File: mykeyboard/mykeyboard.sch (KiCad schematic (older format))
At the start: 2 parts

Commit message: try to select PATH
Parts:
- removed U?: GL850A, symbol Switch:GL850A
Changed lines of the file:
@@
 EESchema Schematic File Version 4
+LIBS:mykeyboard-cache
 EELAYER 26 0
 EELAYER END
@@
 $EndDescr
 $Comp
-L Switch:GL850A U?
-U 1 1 5BE85F64
-P 3000 4200
-F 0 "U?" H 2975 5465 50  0000 C CNN
-F 1 "GL850A" H 2975 5374 50  0000 C CNN
-F 2 "" H 2300 5400 50  0001 C CNN
-F 3 "" H 2300 5400 50  0001 C CNN
-	1    3000 4200
-	1    0    0    -1
-$EndComp
-$Comp
 L MCU_Microchip_ATmega:ATmega32U4-AU U?

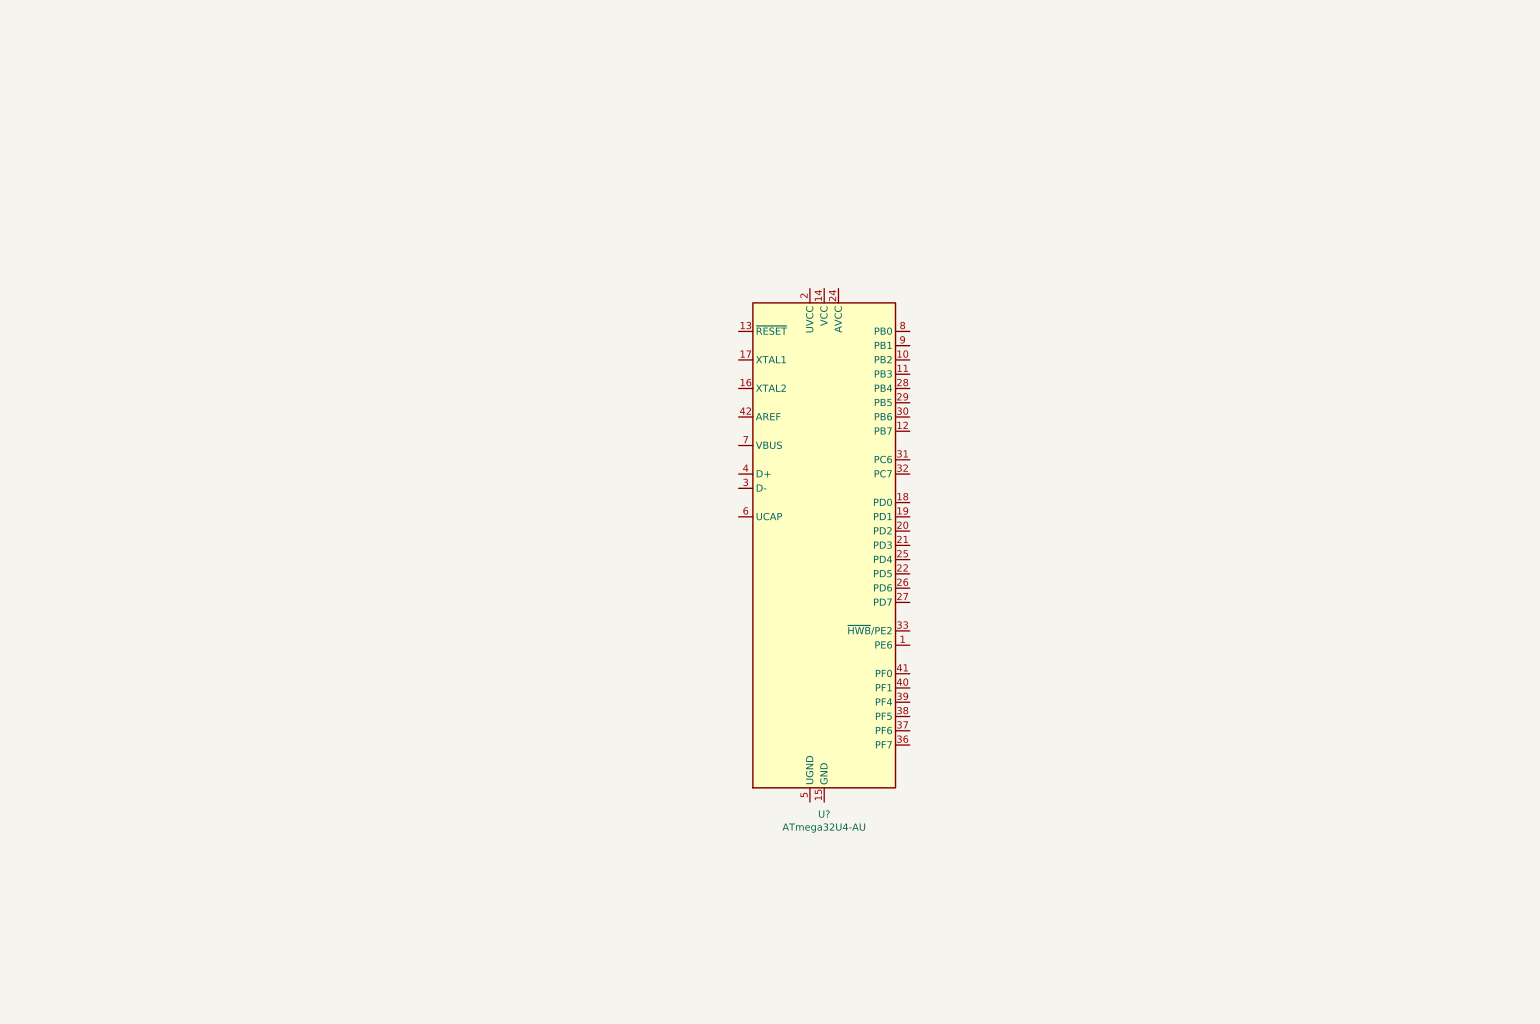
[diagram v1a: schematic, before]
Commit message: 1112,gogogo
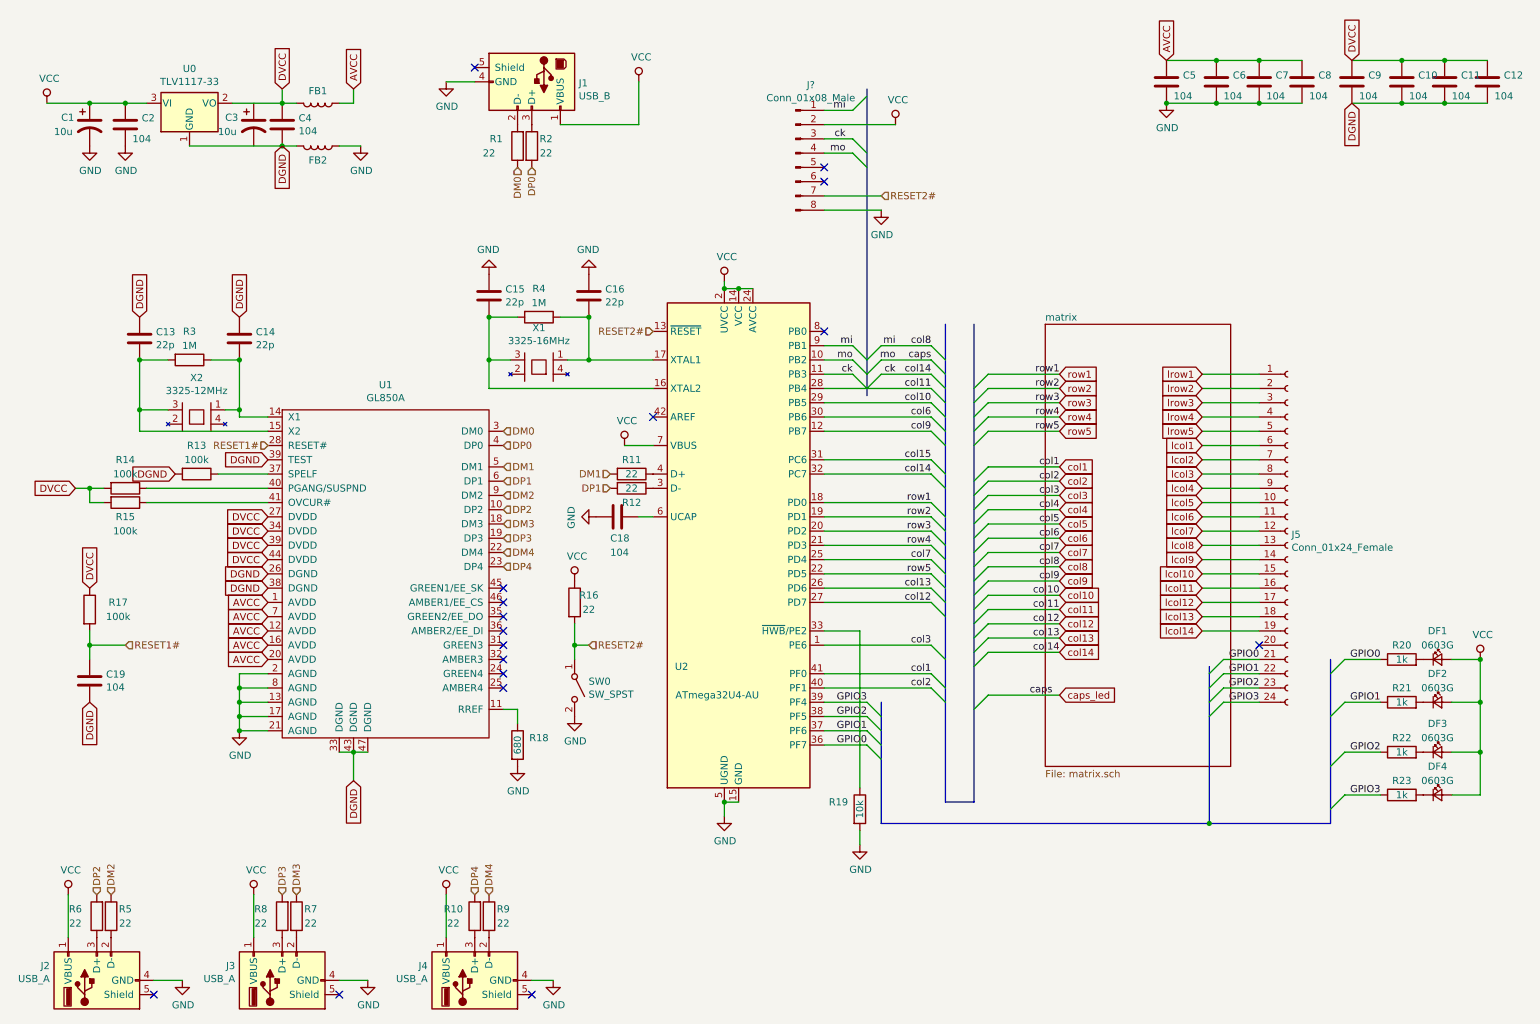
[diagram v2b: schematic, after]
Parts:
- added C1, C3: 10u, symbol Device:CP1
- added C10, C11, C12, C18, C19, C2, C4, C5, C6, C7, C8, C9: 104, symbol Device:C
- added C13, C14, C15, C16: 22p, symbol Device:C
- added DF1, DF2, DF3, DF4: 0603G, symbol Device:LED_Small
- added FB1, FB2: ~, symbol Device:L
- added J1: USB_B, symbol Connector:USB_B
- added J2, J3, J4: USB_A, symbol Connector:USB_A
- added J5: Conn_01x24_Female, symbol Connector:Conn_01x24_Female
- added J?: Conn_01x08_Male, symbol Connector:Conn_01x08_Male
- added R1, R10, R11, R12, R16, R2, R5, R6, R7, R8, R9: 22, symbol Device:R
- added R13, R14, R15, R17: 100k, symbol Device:R
- added R18: 680, symbol Device:R
- added R19: 10k, symbol Device:R
- added R20, R21, R22, R23: 1k, symbol Device:R
- added R3, R4: 1M, symbol Device:R
- added SW0: SW_SPST, symbol Switch:SW_SPST
- added U0: TLV1117-33, symbol Regulator_Linear:TLV1117-33
- added U1: GL850A, symbol mykeyboard-rescue:GL850A-mykeyboardlibs
- added X1: 3325-16MHz, symbol mykeyboard-rescue:3325-16MHz-mykeyboardlibs
- added X2: 3325-12MHz, symbol mykeyboard-rescue:3325-12MHz-mykeyboardlibs
- gave numbers to parts that had none: 1
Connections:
- net col3: now reaches U2.1 (PE6)
- net caps_led: now reaches U2.10 (PB2)
- net caps_led: now also J?.4 (Pin_4)
- net col14: now reaches U2.11 (PB3)
- net col14: now also U2.32 (PC7), J?.3 (Pin_3)
- net col9: now reaches U2.12 (PB7)
- net RESET2#: now reaches U2.13 (~RESET)
- net RESET2#: now also J?.7 (Pin_7), R16.2, SW0.1 (A)
- net VCC: now reaches U2.14 (VCC), U2.34 (VCC)
- net VCC: now also U2.2 (UVCC), U2.24 (AVCC), U2.44 (AVCC), U2.7 (VBUS), C1.1, C2.1, DF1.2 (A), DF2.2 (A), DF3.2 (A), DF4.2 (A), J1.1 (VBUS), J2.1 (VBUS), J3.1 (VBUS), J4.1 (VBUS), J?.2 (Pin_2), R16.1, U0.3 (VI)
- net GND: now reaches U2.15 (GND), U2.23 (GND), U2.35 (GND), U2.43 (GND)
- net GND: now also U2.5 (UGND), C1.2, C15.1, C16.1, C18.2, C2.2, C5.2, C6.2, C7.2, C8.2, FB2.1, J1.4 (GND), J2.4 (GND), J3.4 (GND), J4.4 (GND), J?.8 (Pin_8), R18.2, R19.2, SW0.2 (B), U1.13 (AGND), U1.17 (AGND), U1.2 (AGND), U1.21 (AGND), U1.8 (AGND)
- net at U2.16 (XTAL2): now also C15.2, R4.2, X1.3
- net at U2.17 (XTAL1): now also C16.2, R4.1, X1.1
- net row1: now reaches U2.18 (PD0)
- net row2: now reaches U2.19 (PD1)
- net row3: now reaches U2.20 (PD2)
- net row4: now reaches U2.21 (PD3)
- net row5: now reaches U2.22 (PD5)
- net col7: now reaches U2.25 (PD4)
- net col13: now reaches U2.26 (PD6)
- net col12: now reaches U2.27 (PD7)
- net col11: now reaches U2.28 (PB4)
- net col10: now reaches U2.29 (PB5)
- net at U2.3 (D-): now also R12.1
- net col6: now reaches U2.30 (PB6)
- net col15: now reaches U2.31 (PC6)
- net at U2.33 (~HWB~/PE2): now also R19.1
- net GPIO0: now reaches U2.36 (PF7)
- net GPIO0: now also J5.21 (Pin_21), R20.1
- net GPIO1: now reaches U2.37 (PF6)
- net GPIO1: now also J5.22 (Pin_22), R21.1
- net GPIO2: now reaches U2.38 (PF5)
- net GPIO2: now also J5.23 (Pin_23), R22.1
- net GPIO3: now reaches U2.39 (PF4)
- net GPIO3: now also J5.24 (Pin_24), R23.1
- net at U2.4 (D+): now also R11.1
- net col2: now reaches U2.40 (PF1)
- net col1: now reaches U2.41 (PF0)
- net at U2.6 (UCAP): now also C18.1
- net col8: now reaches U2.9 (PB1)
- net col8: now also J?.1 (Pin_1)
- new net: R18.1, U1.11 (RREF)
- new net: C14.2, R3.1, U1.14 (X1), X2.1
- new net: C13.2, R3.2, U1.15 (X2), X2.3
- new net: R13.1, U1.37 (SPELF)
- new net: R14.1, U1.40 (PGANG/SUSPND)
- new net: R15.1, U1.41 (OVCUR#)
- new net: J1.3 (D+), R2.1
- new net: J1.2 (D-), R1.2
- new net: J2.2 (D-), R5.2
- new net: J2.3 (D+), R6.1
- new net: J3.2 (D-), R7.2
- new net: J3.3 (D+), R8.1
- new net: J4.2 (D-), R9.2
- new net: J4.3 (D+), R10.1
- new net: DF1.1 (K), R20.2
- new net: DF2.1 (K), R21.2
- new net: DF3.1 (K), R22.2
- new net: DF4.1 (K), R23.2
- new net AVCC: C5.1, C6.1, C7.1, C8.1, FB1.1, U1.1 (AVDD), U1.12 (AVDD), U1.16 (AVDD), U1.20 (AVDD), U1.7 (AVDD)
- new net DGND: C10.2, C11.2, C12.2, C13.1, C14.1, C19.2, C4.2, C9.2, FB2.2, R13.2, U0.1 (GND), U1.26 (DGND), U1.33 (DGND), U1.38 (DGND), U1.39 (TEST), U1.43 (DGND), U1.47 (DGND)
- new net DM0: R1.1, U1.3 (DM0)
- new net DM1: R11.2, U1.5 (DM1)
- new net DM2: R5.1, U1.9 (DM2)
- new net DM3: R7.1, U1.18 (DM3)
- new net DM4: R9.1, U1.22 (DM4)
- new net DP0: R2.2, U1.4 (DP0)
- new net DP1: R12.2, U1.6 (DP1)
- new net DP2: R6.2, U1.10 (DP2)
- new net DP3: R8.2, U1.19 (DP3)
- new net DP4: R10.2, U1.23 (DP4)
- new net DVCC: C10.1, C11.1, C12.1, C4.1, C9.1, FB1.2, R14.2, R15.2, R17.1, U0.2 (VO), U1.27 (DVDD), U1.34 (DVDD), U1.39 (TEST), U1.44 (DVDD)
- new net RESET1#: C19.1, R17.2, U1.28 (RESET#)
- new net lcol1: J5.6 (Pin_6)
- new net lcol10: J5.15 (Pin_15)
- new net lcol11: J5.16 (Pin_16)
- new net lcol12: J5.17 (Pin_17)
- new net lcol13: J5.18 (Pin_18)
- new net lcol14: J5.19 (Pin_19)
- new net lcol2: J5.7 (Pin_7)
- new net lcol3: J5.8 (Pin_8)
- new net lcol4: J5.9 (Pin_9)
- new net lcol5: J5.10 (Pin_10)
- new net lcol6: J5.11 (Pin_11)
- new net lcol7: J5.12 (Pin_12)
- new net lcol8: J5.13 (Pin_13)
- new net lcol9: J5.14 (Pin_14)
- new net lrow1: J5.1 (Pin_1)
- new net lrow2: J5.2 (Pin_2)
- new net lrow3: J5.3 (Pin_3)
- new net lrow4: J5.4 (Pin_4)
- new net lrow5: J5.5 (Pin_5)
- no-connect marks 0 -> 17
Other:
- moved on the sheet: U2
